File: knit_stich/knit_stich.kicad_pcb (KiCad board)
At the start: 4 copper layers, 37.8 x 29 mm, 1 part, among them J1 Conn_02x03_Counter_Clockwise

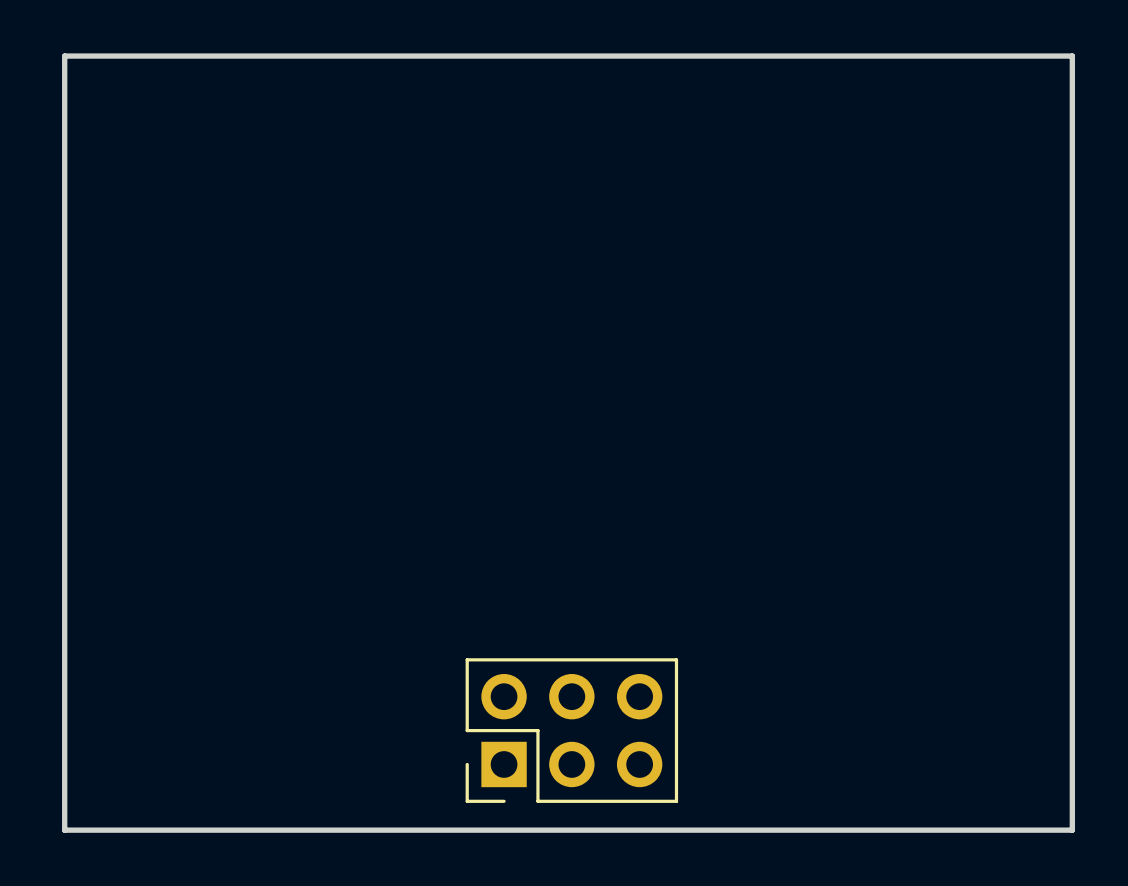
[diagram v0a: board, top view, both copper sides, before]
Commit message: add gitignore
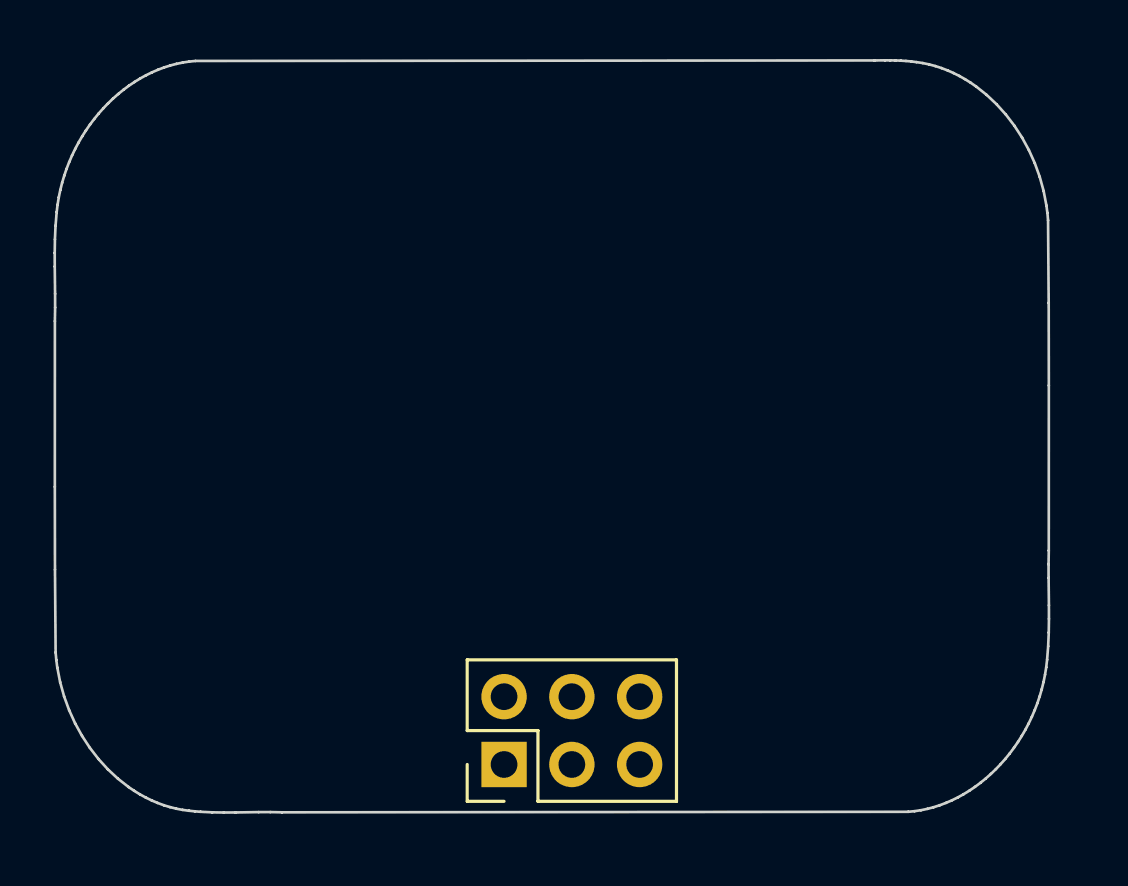
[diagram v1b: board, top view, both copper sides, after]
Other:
- board size 37.8 x 29 mm -> 37.2 x 28.2 mm
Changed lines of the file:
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@@
 		(layer "In2.Cu")
 	)
-	(gr_rect
-		(start 141.75 79.25)
-		(end 179.5 108.25)
+	(gr_poly
+		(pts
+			(xy 172.679214 79.411041) (xy 172.875432 79.414604) (xy 173.071511 79.422028) (xy 173.267372 79.434237)
+			(xy 173.462933 79.452156) (xy 173.658117 79.476708) (xy 173.897271 79.513147) (xy 174.133793 79.562787)
+			(xy 174.367398 79.62527) (xy 174.597799 79.700233) (xy 174.824712 79.787317) (xy 175.047851 79.886162)
+			(xy 175.26693 79.996407) (xy 175.481665 80.117691) (xy 175.691769 80.249654) (xy 175.896958 80.391936)
+			(xy 176.291446 80.706013) (xy 176.662846 81.057038) (xy 177.008873 81.442129) (xy 177.327244 81.858401)
+			(xy 177.615676 82.302971) (xy 177.871885 82.772955) (xy 178.093586 83.26547) (xy 178.278498 83.777631)
+			(xy 178.424335 84.306555) (xy 178.528814 84.849359) (xy 178.56483 85.125065) (xy 178.589651 85.403159)
+			(xy 178.613704 88.496238) (xy 178.619149 91.589729) (xy 178.616918 97.776849) (xy 178.60883 98.288336)
+			(xy 178.610099 98.800184) (xy 178.6221 99.824176) (xy 178.62353 100.335926) (xy 178.615711 100.847252)
+			(xy 178.593993 101.357955) (xy 178.553724 101.867841) (xy 178.521001 102.148441) (xy 178.476622 102.425766)
+			(xy 178.420916 102.699481) (xy 178.354209 102.969252) (xy 178.276828 103.234744) (xy 178.189101 103.495622)
+			(xy 178.091355 103.751553) (xy 177.983917 104.0022) (xy 177.867115 104.247229) (xy 177.741275 104.486307)
+			(xy 177.606726 104.719097) (xy 177.463793 104.945266) (xy 177.312806 105.164479) (xy 177.154089 105.3764)
+			(xy 176.987972 105.580697) (xy 176.814781 105.777032) (xy 176.634843 105.965073) (xy 176.448486 106.144485)
+			(xy 176.256036 106.314932) (xy 176.057822 106.47608) (xy 175.85417 106.627595) (xy 175.645408 106.769142)
+			(xy 175.431862 106.900385) (xy 175.213861 107.020991) (xy 174.99173 107.130625) (xy 174.765799 107.228952)
+			(xy 174.536393 107.315638) (xy 174.30384 107.390347) (xy 174.068467 107.452746) (xy 173.830602 107.502499)
+			(xy 173.590572 107.539272) (xy 173.348703 107.56273) (xy 149.886782 107.582055) (xy 149.452176 107.573133)
+			(xy 149.017336 107.574194) (xy 148.147458 107.587189) (xy 147.712674 107.589587) (xy 147.278161 107.582895)
+			(xy 146.844046 107.562343) (xy 146.627177 107.54538) (xy 146.410456 107.523164) (xy 146.16854 107.491112)
+			(xy 145.929226 107.445427) (xy 145.692807 107.386484) (xy 145.459575 107.314657) (xy 145.229822 107.230323)
+			(xy 145.003841 107.133856) (xy 144.781925 107.025631) (xy 144.564366 106.906024) (xy 144.351456 106.77541)
+			(xy 144.143487 106.634164) (xy 143.743546 106.321276) (xy 143.36688 105.970361) (xy 143.01583 105.584423)
+			(xy 142.692736 105.166461) (xy 142.399936 104.719477) (xy 142.139771 104.246473) (xy 141.91458 103.75045)
+			(xy 141.726703 103.234409) (xy 141.578479 102.701352) (xy 141.472247 102.154281) (xy 141.43561 101.876428)
+			(xy 141.410348 101.596196) (xy 141.386236 98.492292) (xy 141.380784 95.387969) (xy 141.383024 89.179183)
+			(xy 141.391341 88.668768) (xy 141.390029 88.157937) (xy 141.377779 87.135922) (xy 141.376471 86.625182)
+			(xy 141.384794 86.114917) (xy 141.407563 85.60535) (xy 141.449593 85.096702) (xy 141.4835 84.817278)
+			(xy 141.52895 84.541165) (xy 141.58562 84.268691) (xy 141.653185 84.000187) (xy 141.731321 83.735983)
+			(xy 141.819704 83.476408) (xy 141.91801 83.221793) (xy 142.025914 82.972468) (xy 142.143093 82.728762)
+			(xy 142.269222 82.491005) (xy 142.403978 82.259529) (xy 142.547036 82.034661) (xy 142.698073 81.816733)
+			(xy 142.856763 81.606075) (xy 143.022784 81.403016) (xy 143.19581 81.207886) (xy 143.375518 81.021016)
+			(xy 143.561584 80.842735) (xy 143.753683 80.673374) (xy 143.951492 80.513261) (xy 144.154687 80.362728)
+			(xy 144.362942 80.222104) (xy 144.575935 80.091719) (xy 144.793341 79.971903) (xy 145.014836 79.862987)
+			(xy 145.240096 79.765299) (xy 145.468797 79.679171) (xy 145.700614 79.604931) (xy 145.935224 79.542911)
+			(xy 146.172303 79.493439) (xy 146.411526 79.456847) (xy 146.652569 79.433463) (xy 172.090525 79.414254)
+			(xy 172.090513 79.414273) (xy 172.482935 79.410414)
+		)
 		(stroke
-			(width 0.2)
+			(width 0.1)
 			(type solid)
+			(color 255 85 85 1)
 		)
 		(fill no)
@@
 		)
 	)
+	(group ""
+		(members "df4445b0-fc9c-452b-98b0-ab519abb0a29")
+	)
 	(embedded_fonts no)
